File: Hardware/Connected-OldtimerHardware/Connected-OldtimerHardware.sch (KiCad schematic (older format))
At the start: 25 parts, among them J1 CAN_Bus_Connector, J2 MainConnector, J3 NextionConnector, J4 AUXConnector, Q1 2N3906, U1 ParticleElectron, U2 TSR_2-2450, U3 CANTranceiverModule, U4 AdafruitFRAM, U5 AdafruitUltimateGPS, U6 MotionSensor, U7 SFH618A-2

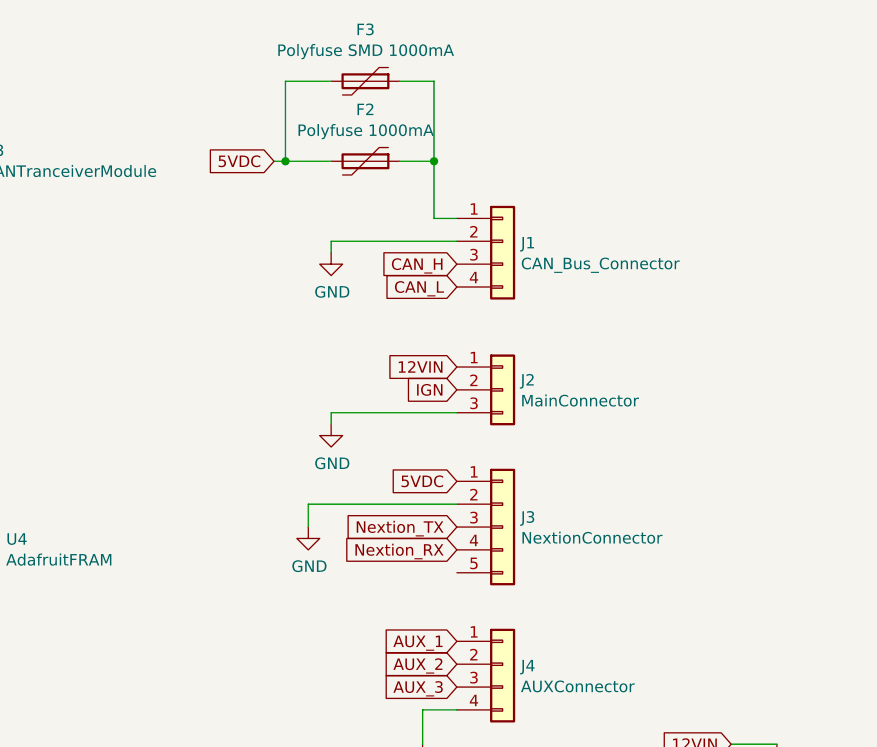
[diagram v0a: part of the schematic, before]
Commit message: changed up connectors
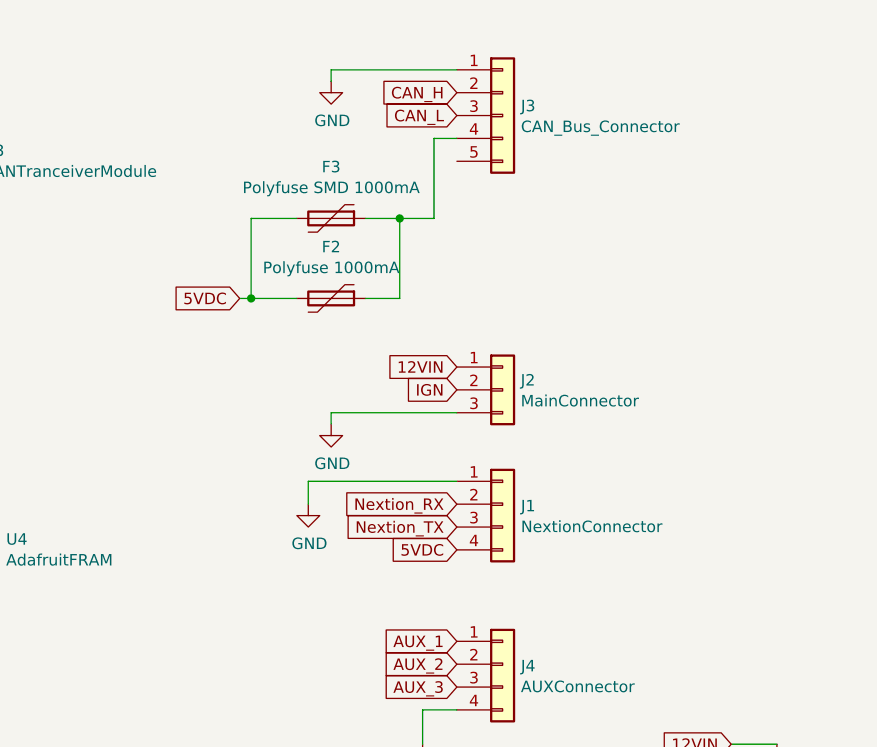
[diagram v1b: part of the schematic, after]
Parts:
- J1: value CAN_Bus_Connector -> NextionConnector; footprint Connector_JST:JST_XH_B04B-XH-A_1x04_P2.50mm_Vertical -> Connector_JST:JST_XH_S04B-XH-A-1_1x04_P2.50mm_Horizontal
- J3: value NextionConnector -> CAN_Bus_Connector; footprint Connector_JST:JST_XH_S05B-XH-A-1_1x05_P2.50mm_Horizontal -> Connector_JST:JST_XH_B05B-XH-A_1x05_P2.50mm_Vertical
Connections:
- net 5VDC: now also J1.4 (Pin_4); no longer J3.1 (Pin_1)
- net CAN_H: now also J3.2 (Pin_2); no longer J1.3 (Pin_3)
- net CAN_L: now also J3.3 (Pin_3); no longer J1.4 (Pin_4)
- net GND: now also J1.1 (Pin_1), J3.1 (Pin_1); no longer J1.2 (Pin_2), J3.2 (Pin_2)
- net Nextion_RX: now also J1.2 (Pin_2); no longer J3.4 (Pin_4)
- net Nextion_TX: now also J1.3 (Pin_3); no longer J3.3 (Pin_3)
- net at F2.1, F3.1: now also J3.4 (Pin_4); no longer J1.1 (Pin_1)
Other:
- moved on the sheet: F2, F3, J1, J3
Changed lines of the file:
@@
 L Connector_Generic:Conn_01x04 J1
 U 1 1 5D676AB8
-P 7250 1550
-F 0 "J1" H 7330 1542 50  0000 L CNN
-F 1 "CAN_Bus_Connector" H 7330 1451 50  0000 L CNN
-F 2 "Connector_JST:JST_XH_B04B-XH-A_1x04_P2.50mm_Vertical" H 7250 1550 50  0001 C CNN
-F 3 "~" H 7250 1550 50  0001 C CNN
-	1    7250 1550
-	1    0    0    -1
-$EndComp
-Text GLabel 6250 1200 0    50   Input ~ 0
+P 7250 2700
+F 0 "J1" H 7330 2692 50  0000 L CNN
+F 1 "NextionConnector" H 7330 2601 50  0000 L CNN
+F 2 "Connector_JST:JST_XH_S04B-XH-A-1_1x04_P2.50mm_Horizontal" H 7250 2700 50  0001 C CNN
+F 3 "~" H 7250 2700 50  0001 C CNN
+	1    7250 2700
+	1    0    0    -1
+$EndComp
+Text GLabel 6100 1800 0    50   Input ~ 0
 5VDC
-Text GLabel 7050 1650 0    50   Input ~ 0
+Text GLabel 7050 900  0    50   Input ~ 0
 CAN_H
-Text GLabel 7050 1750 0    50   Input ~ 0
+Text GLabel 7050 1000 0    50   Input ~ 0
 CAN_L
 Text GLabel 7100 5200 0    50   Input ~ 0
@@
 Text GLabel 7050 2200 0    50   Input ~ 0
 IGN
-Text GLabel 7050 2600 0    50   Input ~ 0
+Text GLabel 7050 2900 0    50   Input ~ 0
 5VDC
 Text GLabel 7050 2800 0    50   Input ~ 0
 Nextion_TX
-Text GLabel 7050 2900 0    50   Input ~ 0
+Text GLabel 7050 2700 0    50   Input ~ 0
 Nextion_RX
 $Comp
@@
 L Connector_Generic:Conn_01x05 J3
 U 1 1 5D6E0A2B
-P 7250 2800
-F 0 "J3" H 7330 2842 50  0000 L CNN
-F 1 "NextionConnector" H 7330 2751 50  0000 L CNN
-F 2 "Connector_JST:JST_XH_S05B-XH-A-1_1x05_P2.50mm_Horizontal" H 7250 2800 50  0001 C CNN
-F 3 "~" H 7250 2800 50  0001 C CNN
-	1    7250 2800
+P 7250 1000
+F 0 "J3" H 7330 1042 50  0000 L CNN
+F 1 "CAN_Bus_Connector" H 7330 951 50  0000 L CNN
+F 2 "Connector_JST:JST_XH_B05B-XH-A_1x05_P2.50mm_Vertical" H 7250 1000 50  0001 C CNN
+F 3 "~" H 7250 1000 50  0001 C CNN
+	1    7250 1000
 	1    0    0    -1
 $EndComp
@@
 L power:GND #PWR0107
 U 1 1 5D6E50E1
-P 6500 1600
-F 0 "#PWR0107" H 6500 1350 50  0001 C CNN
-F 1 "GND" H 6505 1427 50  0000 C CNN
-F 2 "" H 6500 1600 50  0001 C CNN
-F 3 "" H 6500 1600 50  0001 C CNN
-	1    6500 1600
+P 6500 850
+F 0 "#PWR0107" H 6500 600 50  0001 C CNN
+F 1 "GND" H 6505 677 50  0000 C CNN
+F 2 "" H 6500 850 50  0001 C CNN
+F 3 "" H 6500 850 50  0001 C CNN
+	1    6500 850
 	1    0    0    -1
 $EndComp
@@
 L power:GND #PWR0108
 U 1 1 5D6E5123
-P 6400 2800
-F 0 "#PWR0108" H 6400 2550 50  0001 C CNN
-F 1 "GND" H 6405 2627 50  0000 C CNN
-F 2 "" H 6400 2800 50  0001 C CNN
-F 3 "" H 6400 2800 50  0001 C CNN
-	1    6400 2800
+P 6400 2700
+F 0 "#PWR0108" H 6400 2450 50  0001 C CNN
+F 1 "GND" H 6405 2527 50  0000 C CNN
+F 2 "" H 6400 2700 50  0001 C CNN
+F 3 "" H 6400 2700 50  0001 C CNN
+	1    6400 2700
 	1    0    0    -1
 $EndComp
@@
 	6350 5300 6350 5550
 Wire Wire Line
-	7050 2700 6400 2700
-Wire Wire Line
-	6400 2700 6400 2800
-Wire Wire Line
-	7050 1550 6500 1550
-Wire Wire Line
-	6500 1550 6500 1600
+	7050 2600 6400 2600
+Wire Wire Line
+	6400 2600 6400 2700
+Wire Wire Line
+	7050 800  6500 800
+Wire Wire Line
+	6500 800  6500 850
 $Comp
 L power:GND #PWR0110
@@
 L Device:Polyfuse F2
 U 1 1 5D6EB140
-P 6650 1200
-F 0 "F2" V 6425 1200 50  0000 C CNN
-F 1 "Polyfuse 1000mA" V 6516 1200 50  0000 C CNN
-F 2 "Fuse:Fuse_Littelfuse-LVR200" H 6700 1000 50  0001 L CNN
-F 3 "~" H 6650 1200 50  0001 C CNN
-	1    6650 1200
+P 6500 1800
+F 0 "F2" V 6275 1800 50  0000 C CNN
+F 1 "Polyfuse 1000mA" V 6366 1800 50  0000 C CNN
+F 2 "Fuse:Fuse_Littelfuse-LVR200" H 6550 1600 50  0001 L CNN
+F 3 "~" H 6500 1800 50  0001 C CNN
+	1    6500 1800
 	0    1    1    0
 $EndComp
 Wire Wire Line
-	6500 1200 6300 1200
-Wire Wire Line
-	7050 1450 6950 1450
-Wire Wire Line
-	6950 1450 6950 1200
-Wire Wire Line
-	6950 1200 6800 1200
+	6350 1800 6150 1800
+Wire Wire Line
+	6800 1800 6650 1800
 Wire Wire Line
 	2150 4300 3000 4300
@@
 L Device:Polyfuse F3
 U 1 1 5D6F203B
-P 6650 850
-F 0 "F3" V 6425 850 50  0000 C CNN
-F 1 "Polyfuse SMD 1000mA" V 6516 850 50  0000 C CNN
-F 2 "Capacitor_SMD:C_1210_3225Metric_Pad1.42x2.65mm_HandSolder" H 6700 650 50  0001 L CNN
-F 3 "~" H 6650 850 50  0001 C CNN
-	1    6650 850
+P 6500 1450
+F 0 "F3" V 6275 1450 50  0000 C CNN
+F 1 "Polyfuse SMD 1000mA" V 6366 1450 50  0000 C CNN
+F 2 "Capacitor_SMD:C_1210_3225Metric_Pad1.42x2.65mm_HandSolder" H 6550 1250 50  0001 L CNN
+F 3 "~" H 6500 1450 50  0001 C CNN
+	1    6500 1450
 	0    1    1    0
 $EndComp
 Wire Wire Line
-	6300 850  6300 1200
-Wire Wire Line
-	6300 850  6500 850
-Connection ~ 6300 1200
-Wire Wire Line
-	6300 1200 6250 1200
-Wire Wire Line
-	6800 850  6950 850
-Wire Wire Line
-	6950 850  6950 1200
-Connection ~ 6950 1200
+	6150 1450 6150 1800
+Wire Wire Line
+	6150 1450 6350 1450
+Connection ~ 6150 1800
+Wire Wire Line
+	6150 1800 6100 1800
+Wire Wire Line
+	6650 1450 6800 1450
+Wire Wire Line
+	6800 1450 6800 1800
 $Comp
 L Device:Polyfuse F4
@@
 Text GLabel 1500 2150 0    50   Input ~ 0
 VMON
+Wire Wire Line
+	6950 1450 6800 1450
+Connection ~ 6800 1450
+Wire Wire Line
+	7050 1100 6950 1100
+Wire Wire Line
+	6950 1100 6950 1450
 $EndSCHEMATC
